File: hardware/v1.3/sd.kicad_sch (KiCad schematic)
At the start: 3 parts, among them J6 Micro_SD_Card_Det2, U1 ECP5-CABGA256

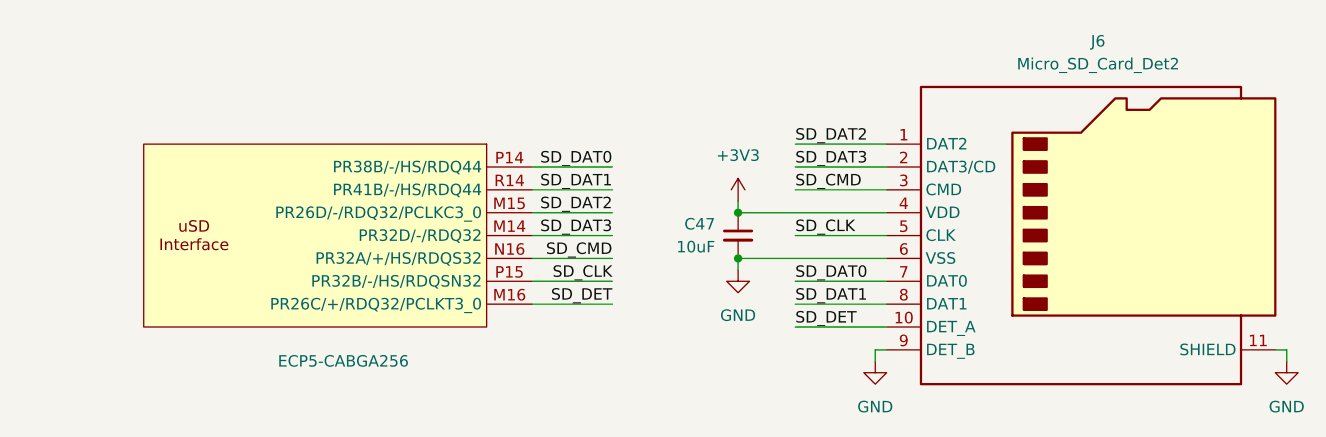
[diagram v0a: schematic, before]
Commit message: Update files
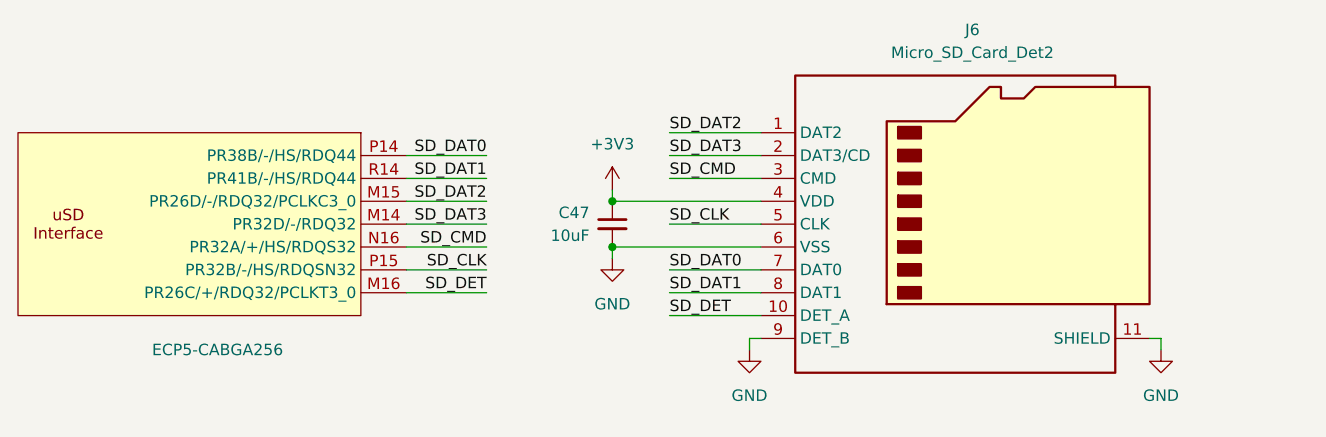
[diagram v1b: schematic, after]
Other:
- moved on the sheet: C47, J6
